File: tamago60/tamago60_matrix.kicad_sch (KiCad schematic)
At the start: 116 parts

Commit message: layout with choc sockets
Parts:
- XSW101, XSW102, XSW103, XSW104, XSW105, XSW106, XSW107, XSW108, XSW109, XSW110, XSW111, XSW112, XSW201, XSW202, XSW203, XSW204, XSW205, XSW206, XSW207, XSW208, XSW209, XSW210, XSW211, XSW212, XSW301, XSW302, XSW303, XSW304, XSW305, XSW306, XSW307, XSW308, XSW309, XSW310, XSW311, XSW312, XSW401, XSW402, XSW403, XSW404, XSW405, XSW406, XSW407, XSW408, XSW409, XSW410, XSW411, XSW412, XSW501, XSW502, XSW503, XSW504, XSW505, XSW508, XSW509, XSW510, XSW511, XSW512: value Kailh MX socket -> Kailh choc socket; footprint tamago60:Kailh_socket_MX -> tamago60:Kailh_socket_PG1350

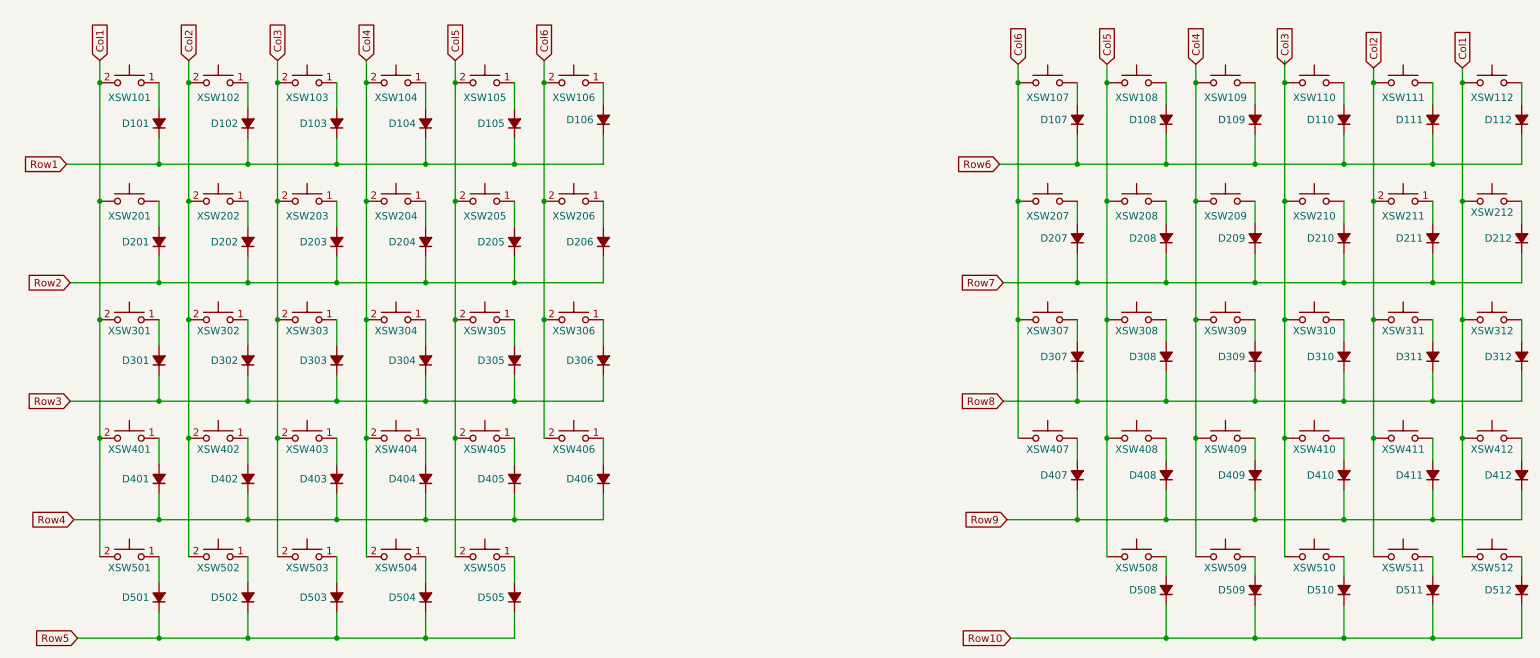
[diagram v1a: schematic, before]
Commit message: routing
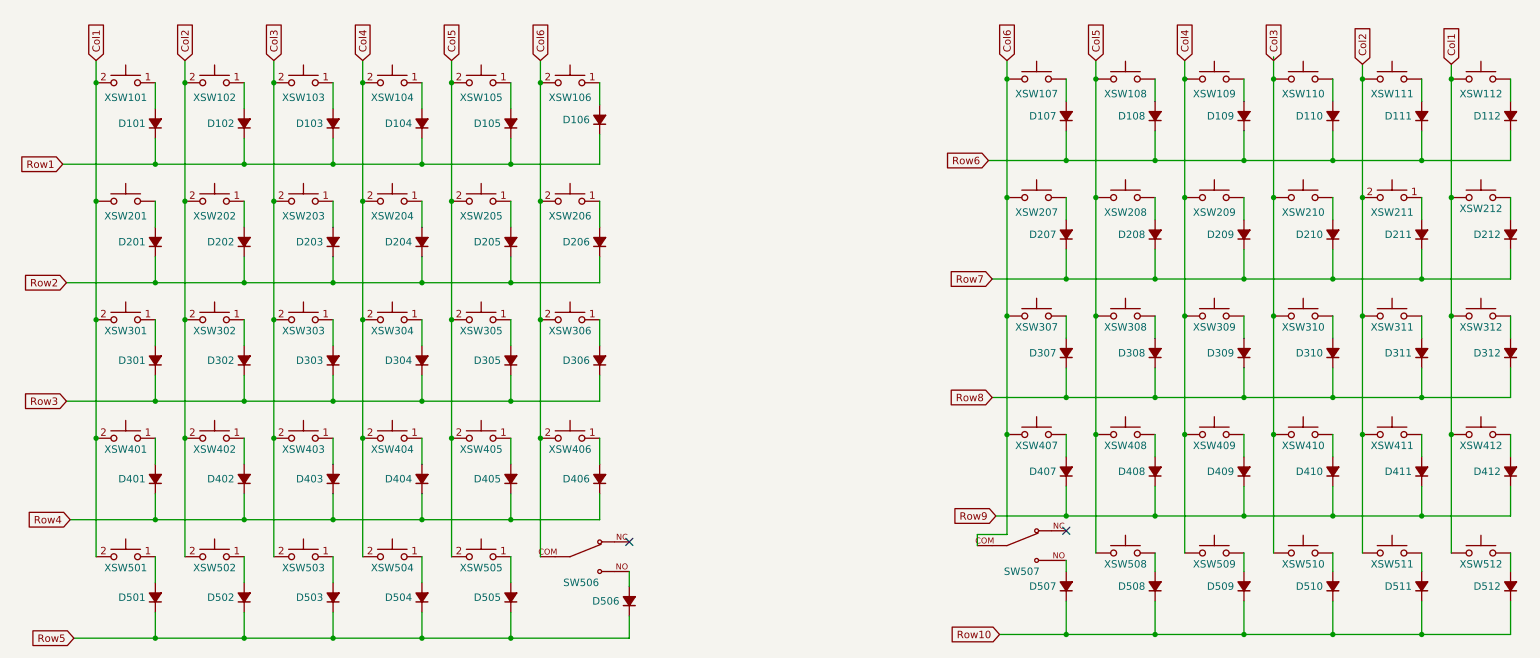
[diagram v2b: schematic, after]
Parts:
- added D506, D507: 1N1418, Diode_SMD:D_SOD-123, symbol Device:D_Small_Filled
- added SW506, SW507: ~, tamago60:SW_D2F-FL, symbol omron_d2f:D2F-FL
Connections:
- net Col6: now also SW506.COM, SW507.COM
- net Row10: now also D507.1 (K)
- net Row5: now also D506.1 (K)
- new net: D506.2 (A), SW506.NO
- new net: D507.2 (A), SW507.NO
- no-connect marks 0 -> 2
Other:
- moved on the sheet: D101, D102, D103, D104, D105, D106, D107, D108, D109, D110, D111, D112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
